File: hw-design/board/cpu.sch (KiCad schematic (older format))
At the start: 11 parts, among them P3 CHAIN, P9 SWD, SW1 SW_PUSH, U3 LPC11U24FBD48/401, Y1 12MHz

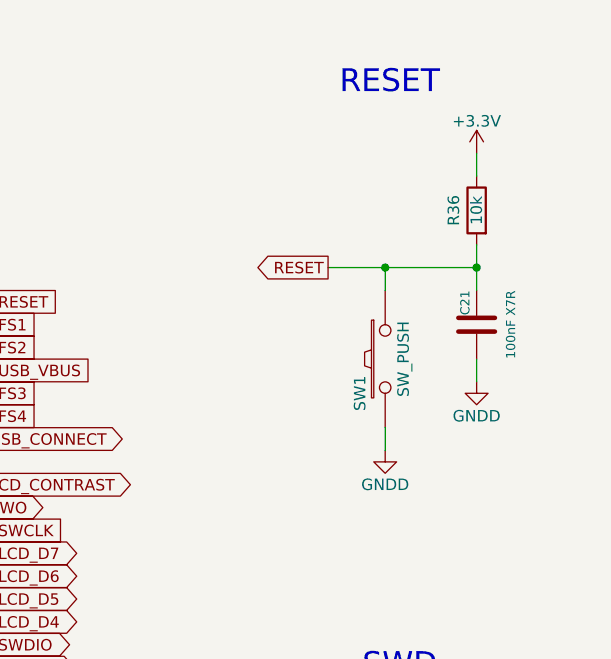
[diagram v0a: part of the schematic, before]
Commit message: replace reset button by pin header
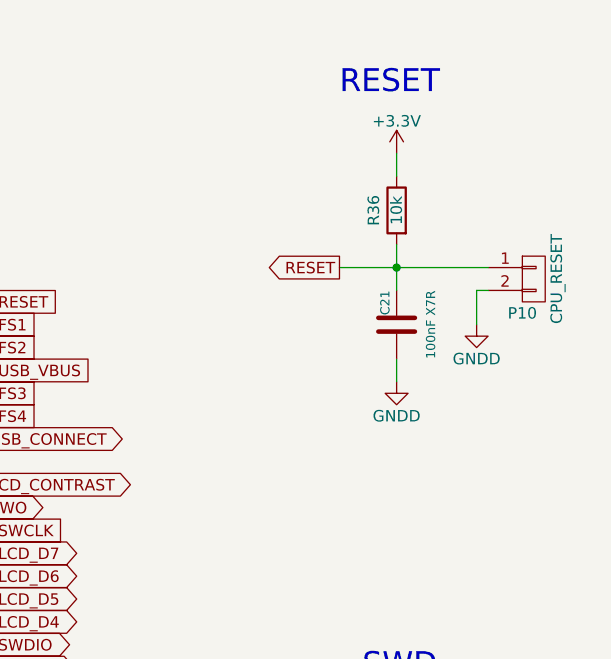
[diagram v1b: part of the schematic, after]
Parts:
- removed SW1: SW_PUSH, Buttons_Switches_SMD:SW_SPST_FSMSM, symbol SW_PUSH
- added P10: CPU_RESET, Pin_Headers:Pin_Header_Straight_1x02, symbol CONN_01X02
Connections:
- net GNDD: now also P10.2 (P2)
- net RESET: now also P10.1 (P1)
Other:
- moved on the sheet: C21, R36

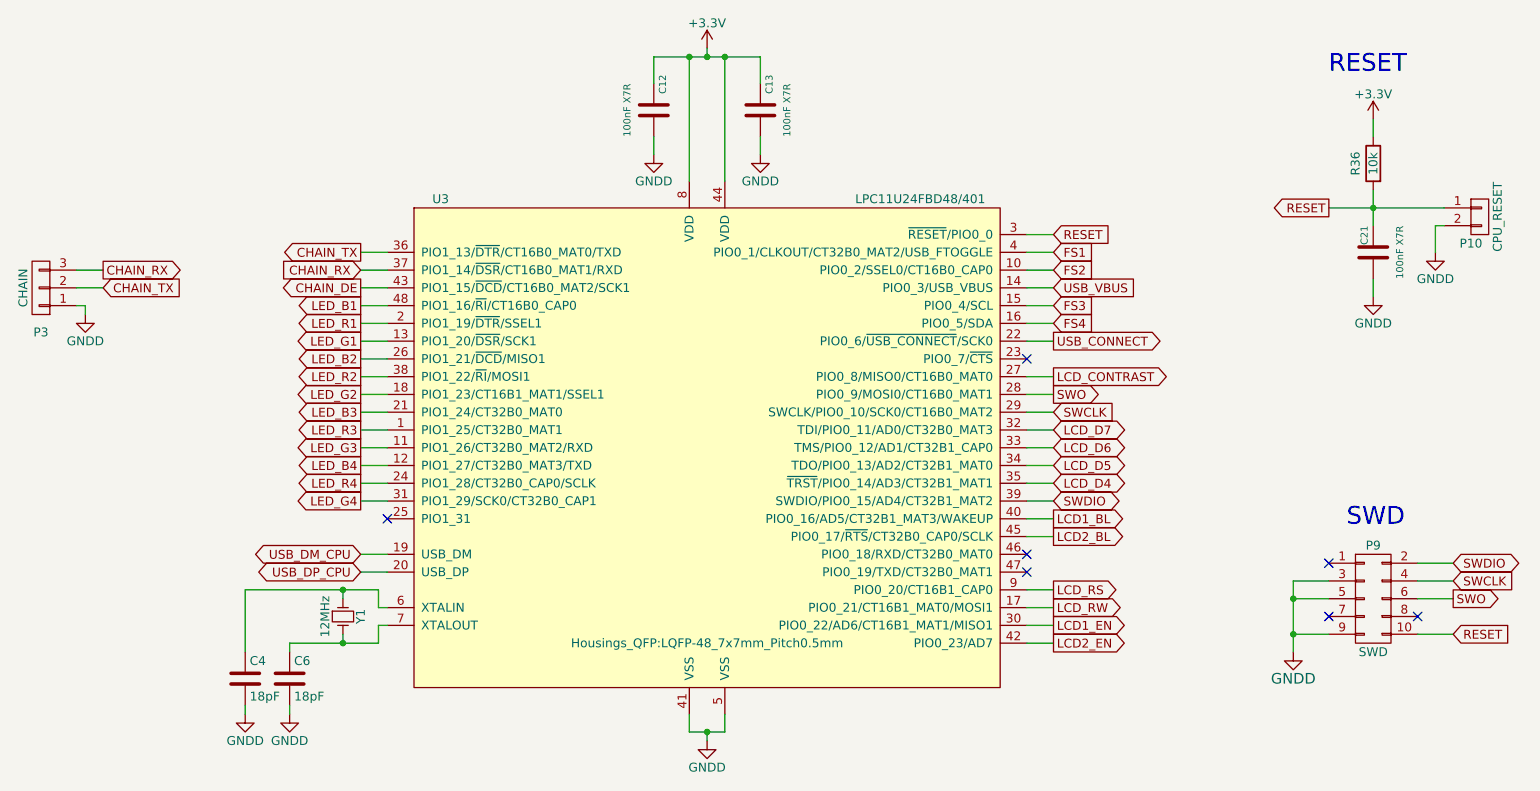
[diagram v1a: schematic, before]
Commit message: fix usb resistors
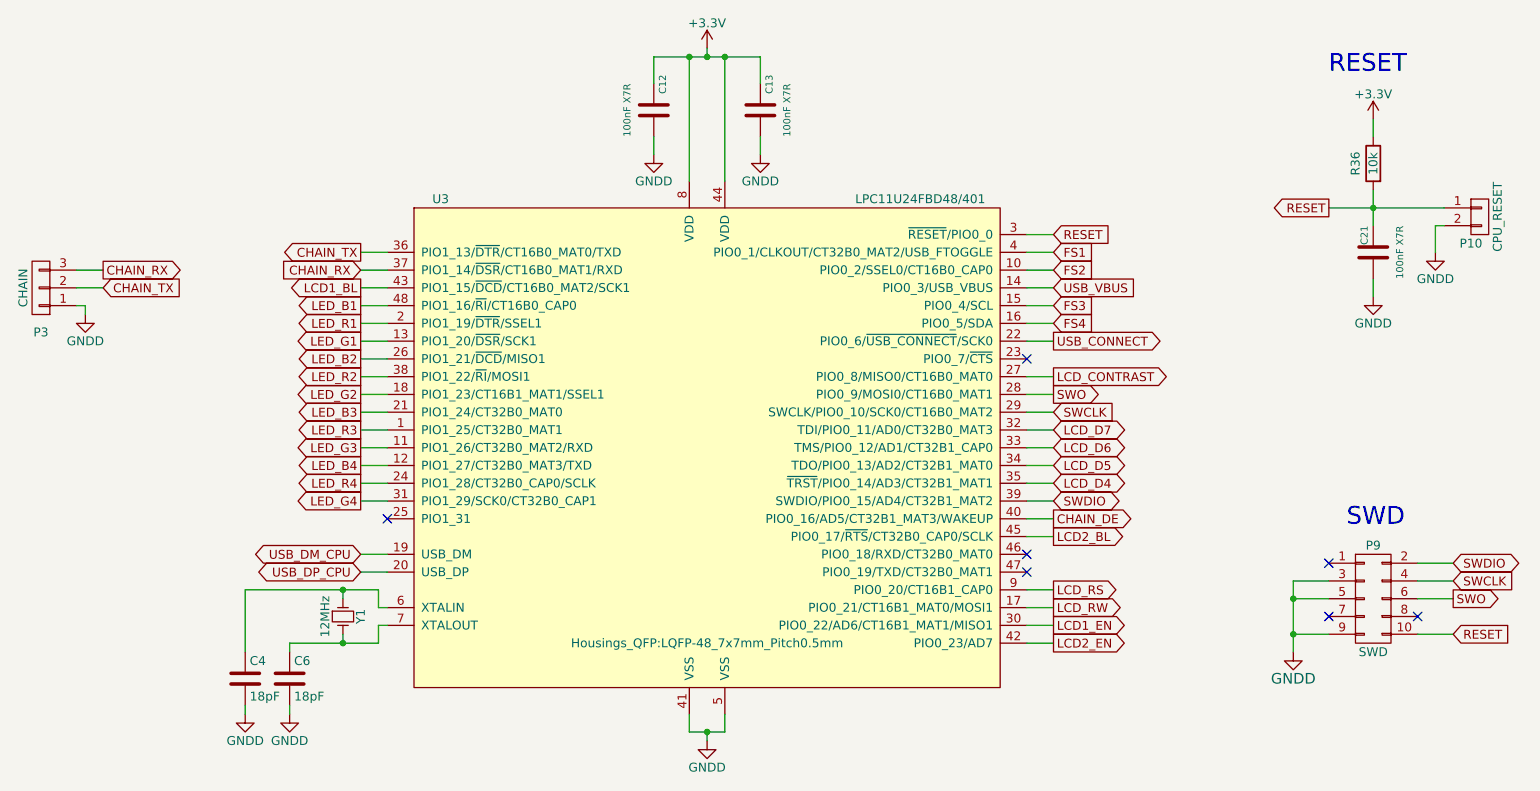
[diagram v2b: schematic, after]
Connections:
- net CHAIN_DE: now also U3.40 (PIO0_16/AD5/CT32B1_MAT3/WAKEUP); no longer U3.43 (PIO1_15/~DCD~/CT16B0_MAT2/SCK1)
- net LCD1_BL: now also U3.43 (PIO1_15/~DCD~/CT16B0_MAT2/SCK1); no longer U3.40 (PIO0_16/AD5/CT32B1_MAT3/WAKEUP)
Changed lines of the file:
@@
 Text GLabel 3600 2750 0    50   Input ~ 0
 CHAIN_RX
-Text GLabel 3600 2850 0    50   Output ~ 0
+Text GLabel 7500 4150 2    50   Output ~ 0
 CHAIN_DE
 Text GLabel 2150 2850 2    50   Input ~ 0
@@
 Text GLabel 7500 4850 2    50   Output ~ 0
 LCD2_EN
-Text GLabel 7500 4150 2    50   Output ~ 0
+Text GLabel 3600 2850 0    50   Output ~ 0
 LCD1_BL
 Text GLabel 7500 4250 2    50   Output ~ 0
@@
 	3600 2750 3750 2750
 Wire Wire Line
-	3750 2850 3600 2850
+	7350 4150 7500 4150
 Wire Wire Line
 	2000 2850 2150 2850
@@
 	7350 3350 7500 3350
 Wire Wire Line
-	7500 4150 7350 4150
+	3600 2850 3750 2850
 Wire Wire Line
 	7350 4250 7500 4250
